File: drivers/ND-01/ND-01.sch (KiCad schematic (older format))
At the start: 0 parts

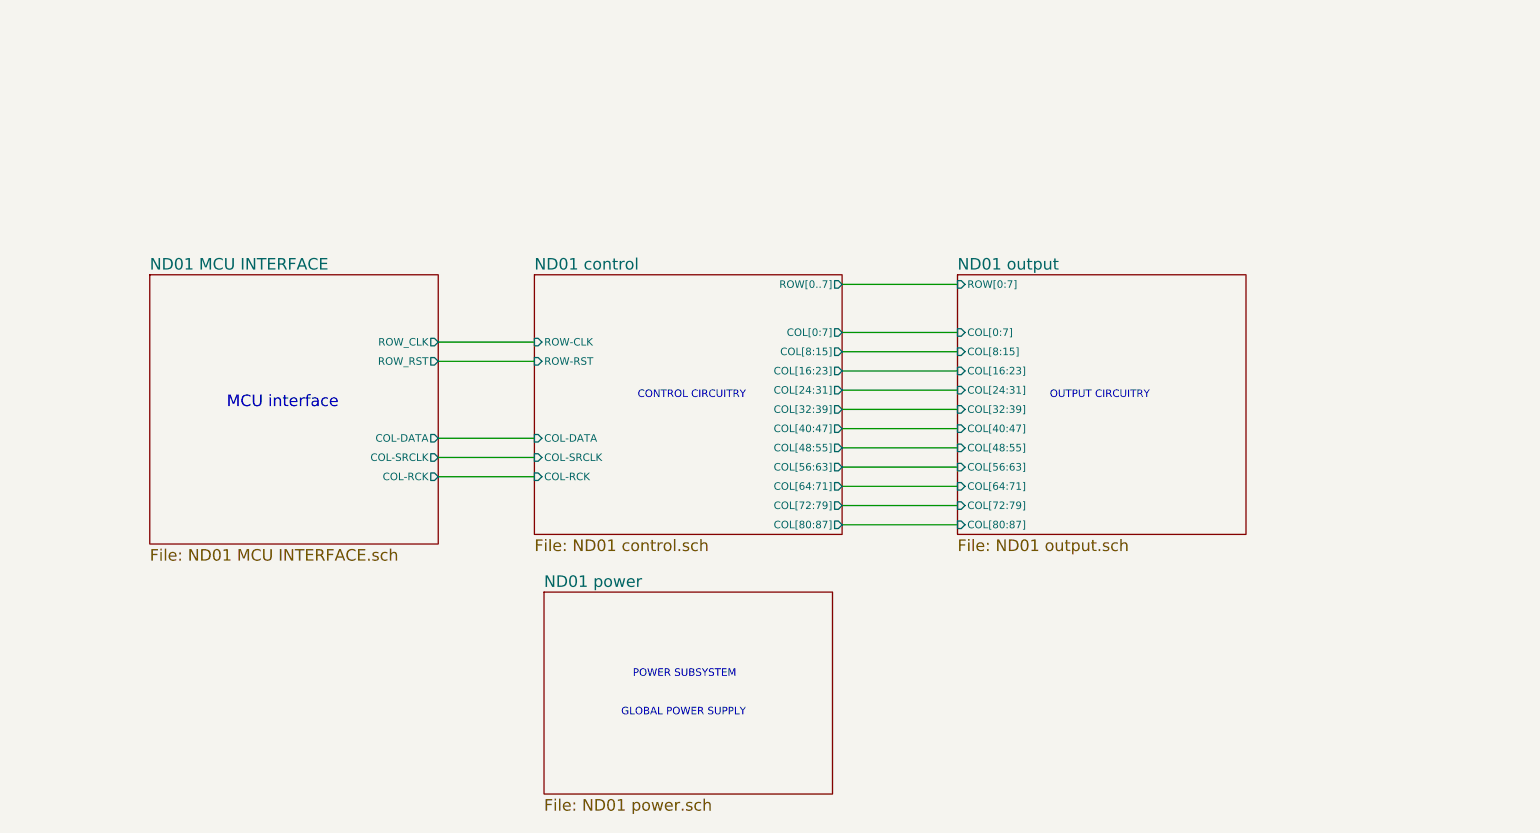
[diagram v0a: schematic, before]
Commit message: Add separate driver uses to schematic
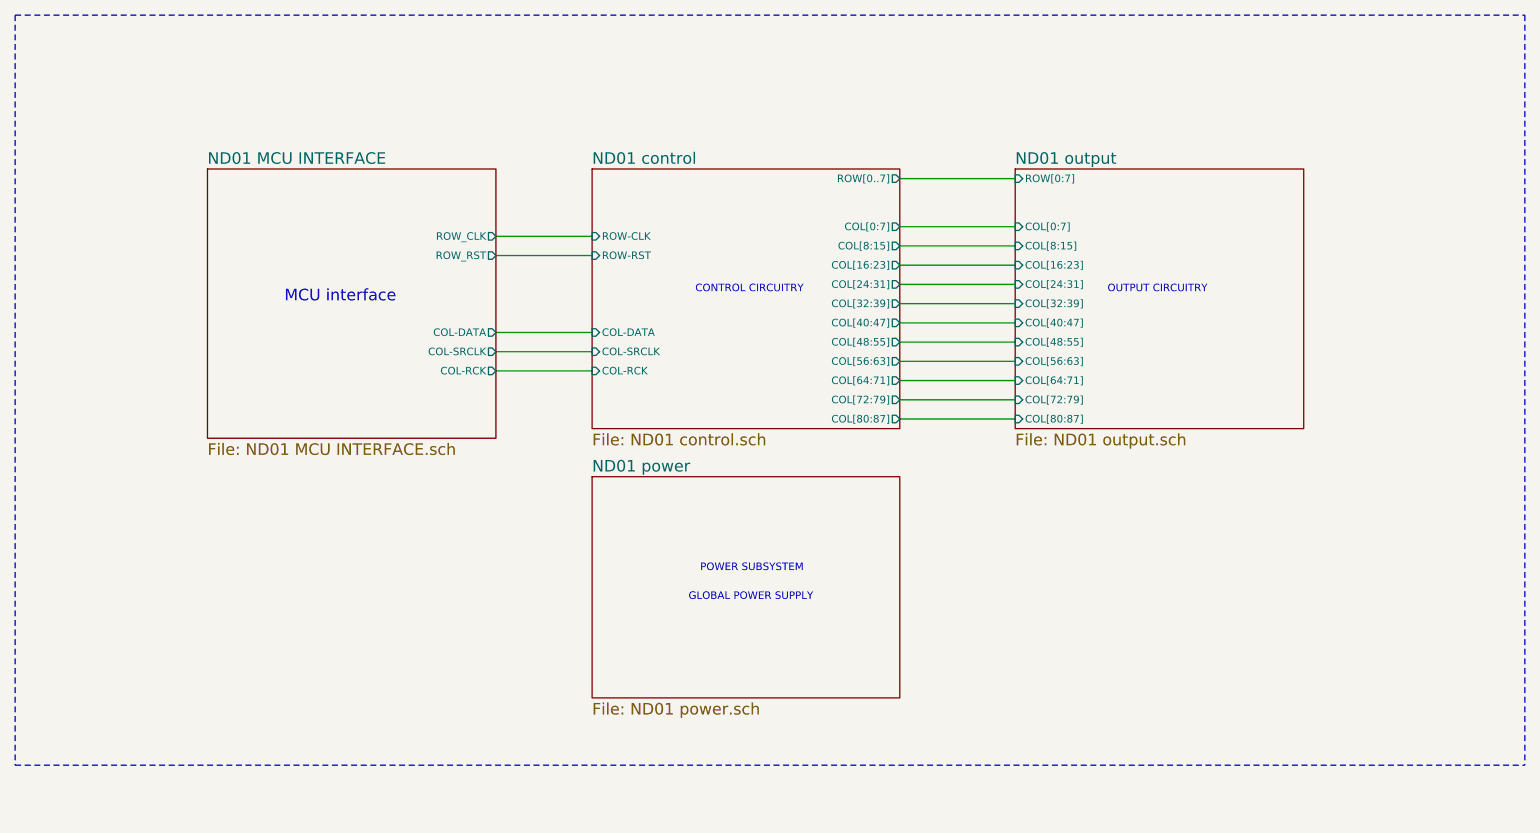
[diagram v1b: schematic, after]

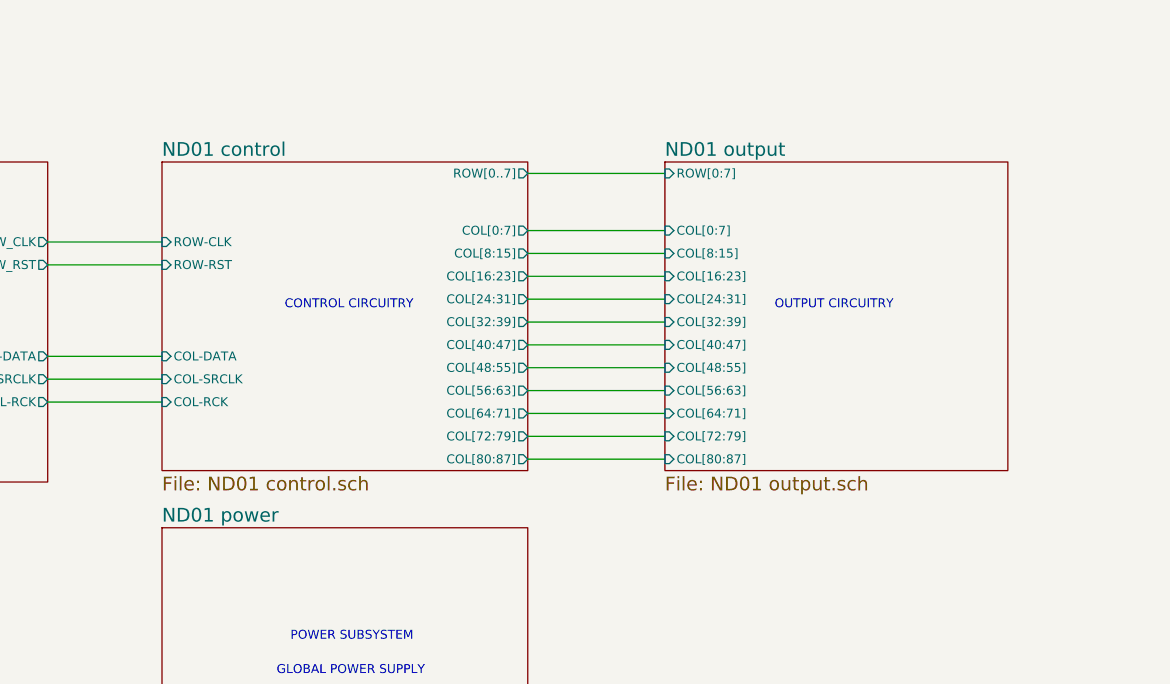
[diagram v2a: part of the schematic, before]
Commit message: semicomplete design
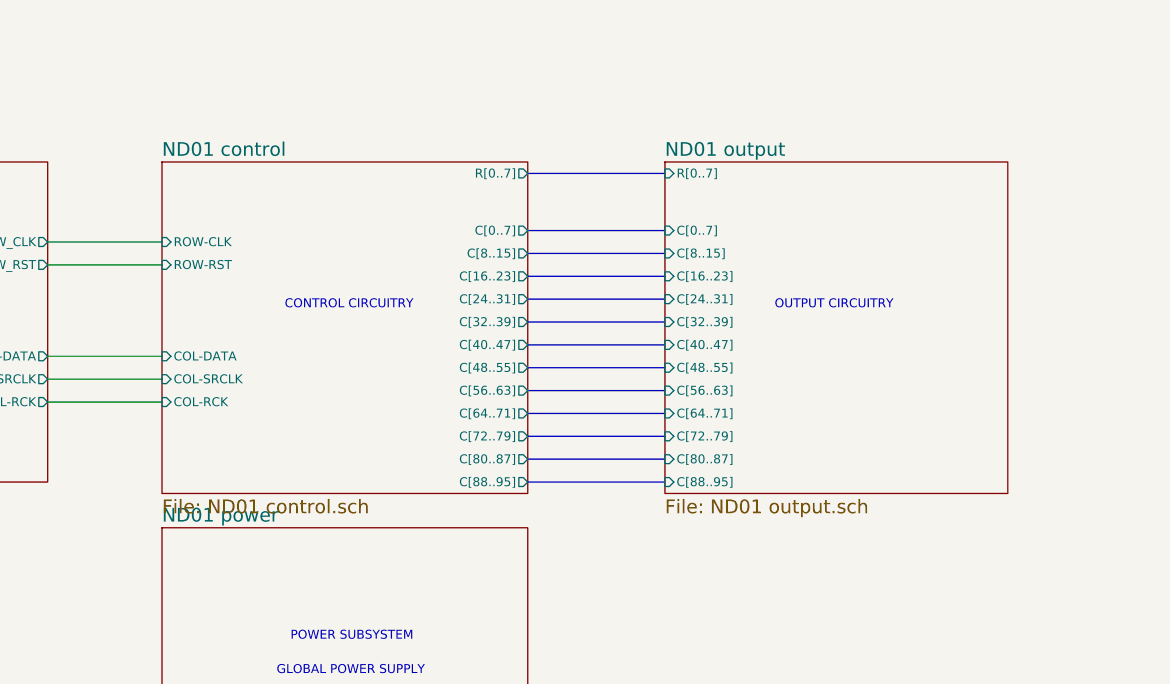
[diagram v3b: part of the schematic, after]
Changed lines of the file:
@@
 F6 "COL-RCK" O R 4400 3850 39
 $EndSheet
-$Sheet
-S 4900 2800 1600 1350
-U 58E5FCE9
-F0 "ND01 control" 60
-F1 "ND01 control.sch" 60
-F2 "ROW[0..7]" O R 6500 2850 39
-F3 "COL[0:7]" O R 6500 3100 39
-F4 "COL-SRCLK" I L 4900 3750 39
-F5 "COL-DATA" I L 4900 3650 39
-F6 "COL[8:15]" O R 6500 3200 39
-F7 "COL[16:23]" O R 6500 3300 39
-F8 "COL[24:31]" O R 6500 3400 39
-F9 "COL[32:39]" O R 6500 3500 39
-F10 "COL[40:47]" O R 6500 3600 39
-F11 "COL[48:55]" O R 6500 3700 39
-F12 "COL[56:63]" O R 6500 3800 39
-F13 "COL[64:71]" O R 6500 3900 39
-F14 "COL[72:79]" O R 6500 4000 39
-F15 "COL[80:87]" O R 6500 4100 39
-F16 "ROW-CLK" I L 4900 3150 39
-F17 "ROW-RST" I L 4900 3250 39
-F18 "COL-RCK" I L 4900 3850 39
-$EndSheet
 Wire Wire Line
 	4400 3150 4900 3150
@@
 Wire Wire Line
 	4400 3850 4900 3850
-Wire Wire Line
-	6500 2850 7100 2850
-$Sheet
-S 7100 2800 1500 1350
-U 58E75CFC
-F0 "ND01 output" 60
-F1 "ND01 output.sch" 60
-F2 "ROW[0:7]" I L 7100 2850 39
-F3 "COL[0:7]" I L 7100 3100 39
-F4 "COL[8:15]" I L 7100 3200 39
-F5 "COL[16:23]" I L 7100 3300 39
-F6 "COL[24:31]" I L 7100 3400 39
-F7 "COL[32:39]" I L 7100 3500 39
-F8 "COL[40:47]" I L 7100 3600 39
-F9 "COL[48:55]" I L 7100 3700 39
-F10 "COL[56:63]" I L 7100 3800 39
-F11 "COL[64:71]" I L 7100 3900 39
-F12 "COL[72:79]" I L 7100 4000 39
-F13 "COL[80:87]" I L 7100 4100 39
-$EndSheet
-Wire Wire Line
-	6500 3100 7100 3100
-Wire Wire Line
-	6500 3200 7100 3200
-Wire Wire Line
-	6500 3300 7100 3300
-Wire Wire Line
-	6500 3400 7100 3400
-Wire Wire Line
-	6500 3500 7100 3500
-Wire Wire Line
-	6500 3600 7100 3600
-Wire Wire Line
-	6500 3700 7100 3700
-Wire Wire Line
-	6500 3800 7100 3800
-Wire Wire Line
-	6500 3900 7100 3900
-Wire Wire Line
-	6500 4000 7100 4000
-Wire Wire Line
-	6500 4100 7100 4100
 Text Notes 3300 3500 0    60   ~ 0
 MCU interface
@@
 Wire Notes Line
 	9750 2000 9750 5900
+Wire Bus Line
+	7100 2850 6500 2850
+Wire Bus Line
+	7100 3100 6500 3100
+Wire Bus Line
+	7100 3200 6500 3200
+Wire Bus Line
+	7100 3300 6500 3300
+Wire Bus Line
+	7100 3400 6500 3400
+Wire Bus Line
+	7100 3500 6500 3500
+Wire Bus Line
+	7100 3600 6500 3600
+Wire Bus Line
+	7100 3700 6500 3700
+Wire Bus Line
+	7100 3800 6500 3800
+Wire Bus Line
+	7100 3900 6500 3900
+Wire Bus Line
+	7100 4000 6500 4000
+Wire Bus Line
+	7100 4100 6500 4100
+Wire Bus Line
+	7100 4200 6500 4200
+$Sheet
+S 4900 2800 1600 1450
+U 58E5FCE9
+F0 "ND01 control" 60
+F1 "ND01 control.sch" 60
+F2 "COL-SRCLK" I L 4900 3750 39
+F3 "COL-DATA" I L 4900 3650 39
+F4 "ROW-CLK" I L 4900 3150 39
+F5 "ROW-RST" I L 4900 3250 39
+F6 "COL-RCK" I L 4900 3850 39
+F7 "C[0..7]" O R 6500 3100 39
+F8 "R[0..7]" O R 6500 2850 39
+F9 "C[8..15]" O R 6500 3200 39
+F10 "C[16..23]" O R 6500 3300 39
+F11 "C[24..31]" O R 6500 3400 39
+F12 "C[32..39]" O R 6500 3500 39
+F13 "C[40..47]" O R 6500 3600 39
+F14 "C[48..55]" O R 6500 3700 39
+F15 "C[56..63]" O R 6500 3800 39
+F16 "C[64..71]" O R 6500 3900 39
+F17 "C[72..79]" O R 6500 4000 39
+F18 "C[80..87]" O R 6500 4100 39
+F19 "C[88..95]" O R 6500 4200 39
+$EndSheet
+$Sheet
+S 7100 2800 1500 1450
+U 58E75CFC
+F0 "ND01 output" 60
+F1 "ND01 output.sch" 60
+F2 "C[0..7]" I L 7100 3100 39
+F3 "C[8..15]" I L 7100 3200 39
+F4 "C[16..23]" I L 7100 3300 39
+F5 "C[24..31]" I L 7100 3400 39
+F6 "C[32..39]" I L 7100 3500 39
+F7 "C[40..47]" I L 7100 3600 39
+F8 "C[48..55]" I L 7100 3700 39
+F9 "C[56..63]" I L 7100 3800 39
+F10 "C[64..71]" I L 7100 3900 39
+F11 "C[72..79]" I L 7100 4000 39
+F12 "C[80..87]" I L 7100 4100 39
+F13 "C[88..95]" I L 7100 4200 39
+F14 "R[0..7]" I L 7100 2850 39
+$EndSheet
 $EndSCHEMATC
